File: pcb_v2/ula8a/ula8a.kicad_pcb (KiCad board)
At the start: 2 copper layers, 165 x 210 mm, 81 parts, among them J1 designador, J2 ula_opp, J3 ula_opp, J4 ula_opp, J5 ula_opp, J6 ula_opp, J7 ula_opp, J8 sysbus_1, J9 sysbus2, Q1 BC548, U1 74LS86, U10 74LS244, U11 74LS86, U12 74LS244, U13 74LS574, U14 74LS00, U15 MC14495P, U16 SA39-11EWA, U17 74LS244, U2 74LS86, U21 74LS244, U22 74LS04, U3 74LS86, U4 74LS86, U5 74LS244, U6 74LS86, U7 74LS86, U8 74LS574, U9 74LS00

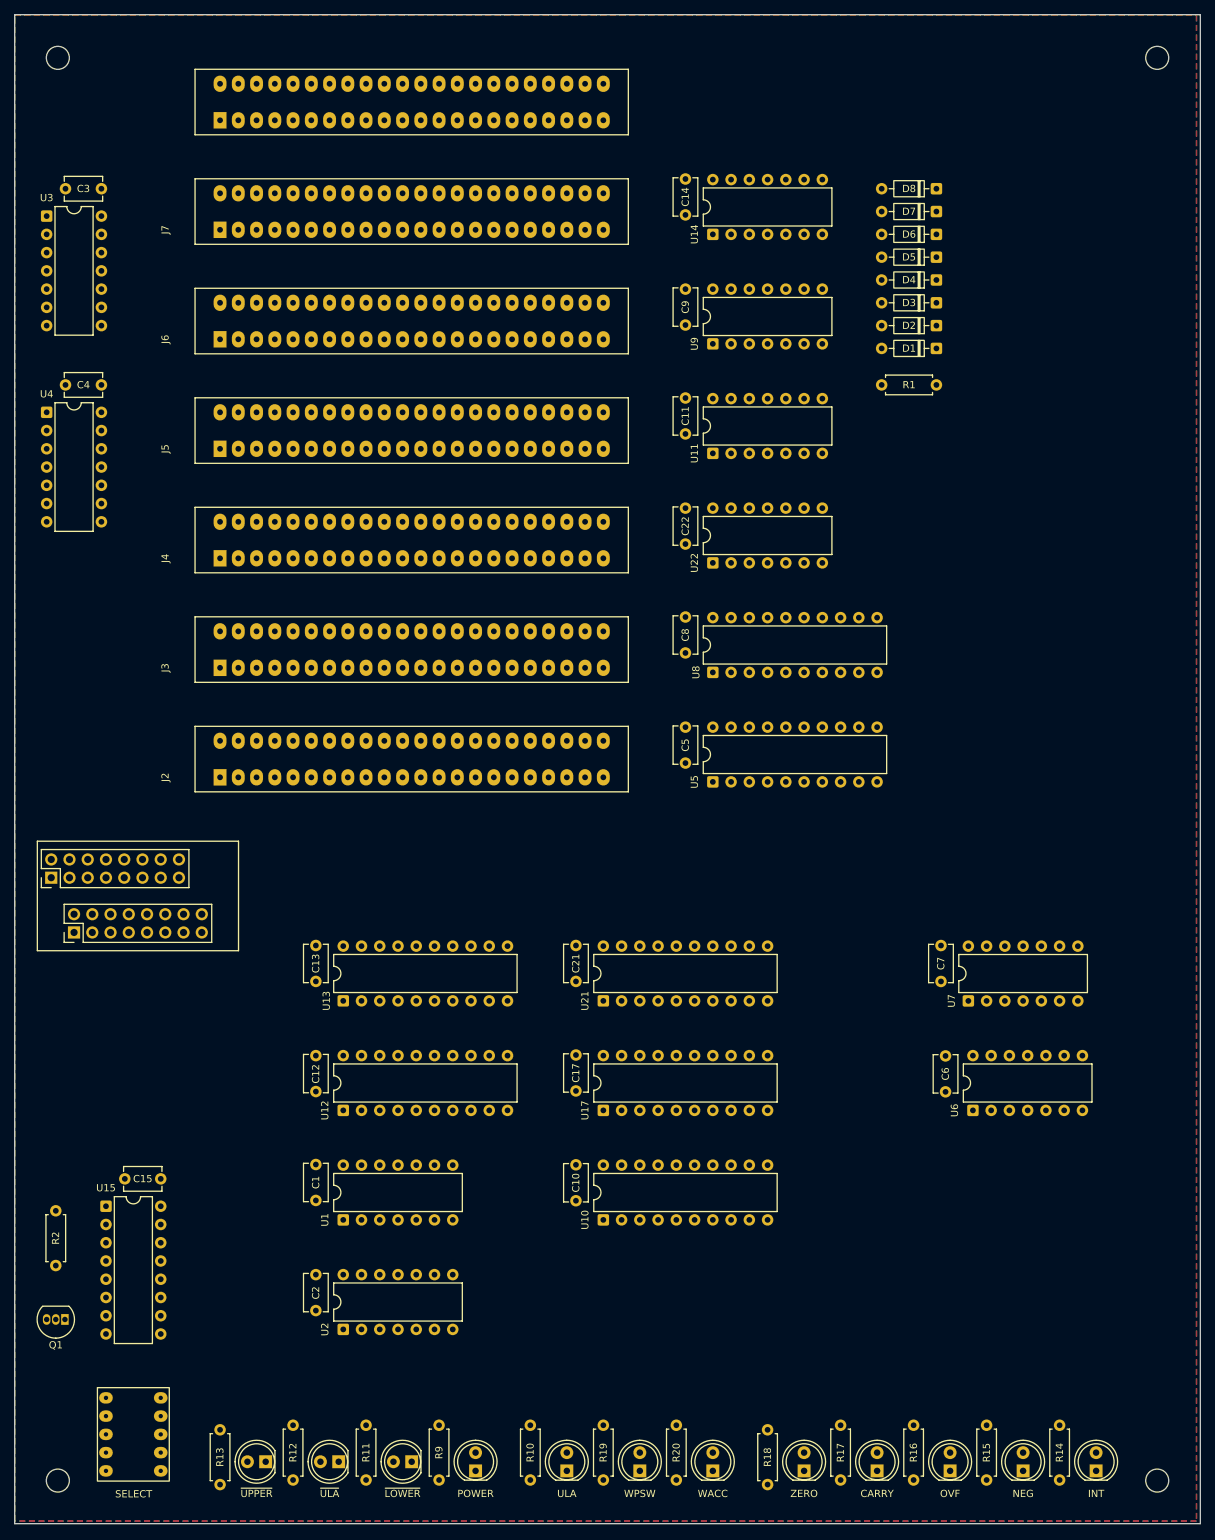
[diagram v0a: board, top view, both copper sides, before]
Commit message: concluído o layout da pcb
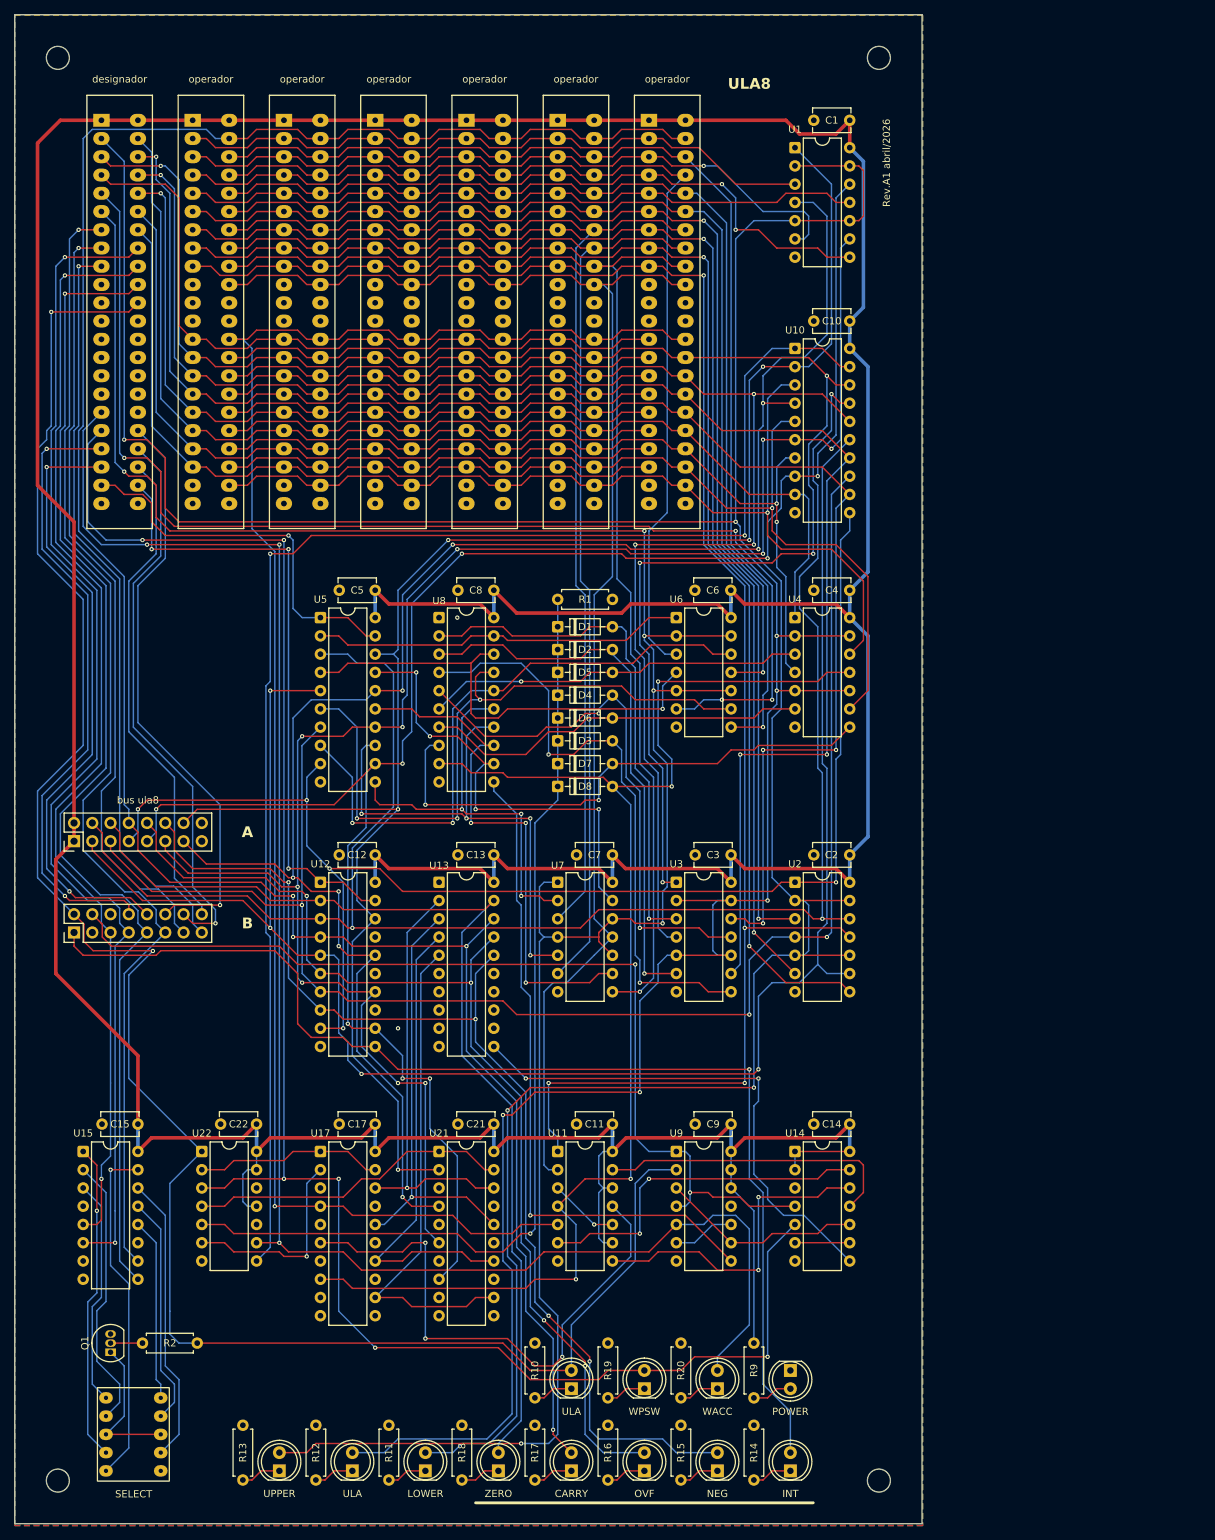
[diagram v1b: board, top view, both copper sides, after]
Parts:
- D11: value ~{LOWER} -> LOWER
- D12: value ~{ULA} -> ULA
- D13: value ~{UPPER} -> UPPER
- J2, J3, J4, J5, J6, J7: value ula_opp -> operador
- J8: value sysbus_1 -> bus_mgrf_1
- J9: value sysbus2 -> bus_mgrf_2
- moved C1 165.5 mm to (124.5, 27.9), turned to 0 degrees
- moved U1 161.9 mm to (121.9, 31.8), turned to 0 degrees
- moved U14 128.1 mm to (121.9, 171.4), turned to 0 degrees
- moved C14 127.8 mm to (124.5, 167.6), turned to 0 degrees
- moved C3 127.6 mm to (108.0, 130.2)
- moved U3 127.6 mm to (105.4, 134.0)
- moved C10 126.8 mm to (124.5, 55.9), turned to 0 degrees
- moved U10 124.2 mm to (121.9, 59.7), turned to 0 degrees
- moved U9 112.5 mm to (105.4, 171.4), turned to 0 degrees
- moved C9 111.2 mm to (108.0, 167.6), turned to 0 degrees
- moved U22 108.5 mm to (39.4, 171.4), turned to 0 degrees
- moved C4 108.0 mm to (124.5, 93.3)
- moved U4 108.0 mm to (121.9, 97.2)
- moved C22 103.4 mm to (42.0, 167.6), turned to 0 degrees
- moved U11 99.5 mm to (88.9, 171.4), turned to 0 degrees
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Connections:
- U6 pad 1: invert_upper_bus -> Net-(U5-I0a)
- U6 pad 10: Net-(U5-I2a) -> invert_upper_bus
- U6 pad 12: invert_upper_bus -> Net-(U5-I3a)
- U6 pad 13: Net-(U5-I3a) -> invert_upper_bus
- U6 pad 2: Net-(U5-I0a) -> invert_upper_bus
- U6 pad 3: upper_bus0 -> upper_bus1
- U6 pad 4: invert_upper_bus -> Net-(U5-I1a)
- U6 pad 5: Net-(U5-I1a) -> invert_upper_bus
- U6 pad 6: upper_bus1 -> upper_bus0
- U6 pad 9: invert_upper_bus -> Net-(U5-I2a)
- U7 pad 10: Net-(U5-I2b) -> invert_upper_bus
- U7 pad 9: invert_upper_bus -> Net-(U5-I2b)
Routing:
- net +5V: track 0.00 -> 744.7 mm
- net invert_lower_bus: track 0.00 -> 411.0 mm, vias 0 -> 4
- net invert_ula_bus: track 0.00 -> 346.6 mm, vias 0 -> 7
- net invert_upper_bus: track 0.00 -> 336.9 mm, vias 0 -> 6
- net carry_flag_out: track 0.00 -> 329.4 mm, vias 0 -> 4
- net ula_enable: track 0.00 -> 274.0 mm, vias 0 -> 2
- net data_3: track 0.00 -> 261.5 mm, vias 0 -> 8
- net data_6: track 0.00 -> 255.2 mm, vias 0 -> 4
- net write_psw: track 0.00 -> 253.7 mm, vias 0 -> 6
- net data_2: track 0.00 -> 251.1 mm, vias 0 -> 10
- net data_1: track 0.00 -> 247.6 mm, vias 0 -> 8
- net data_0: track 0.00 -> 244.4 mm, vias 0 -> 5
- net lower_bus7: track 0.00 -> 244.2 mm, vias 0 -> 4
- net data_7: track 0.00 -> 243.4 mm, vias 0 -> 3
- net write_acc: track 0.00 -> 238.1 mm, vias 0 -> 3
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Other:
- board size 165 x 210 mm -> 126.3 x 210 mm
- board text added: "A"
- board text added: "B"
- board text added: "Rev.A1 abril/2026"
- board text added: "ULA8"
- board text added: "bus ula8"
